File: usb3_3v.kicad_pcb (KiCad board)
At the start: 2 copper layers, 6 parts, among them J1 USB-MICRO-B, P1 +3.3, P2 GND, U1 AAT3221 / MIC5504

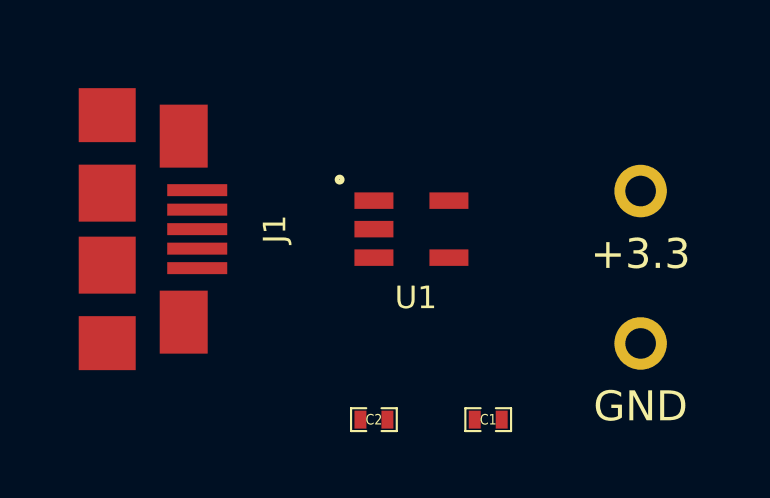
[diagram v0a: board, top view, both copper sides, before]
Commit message: - pcb done, add gerbers
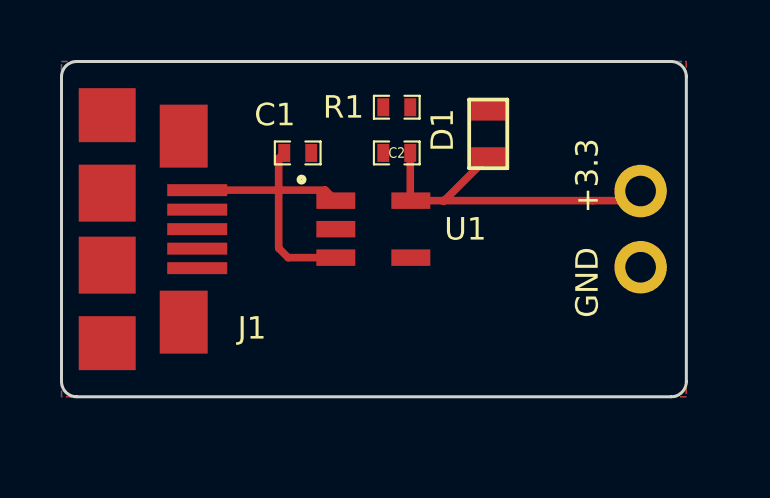
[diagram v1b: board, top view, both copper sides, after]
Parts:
- added D1: LED, SM0603, F.Cu at (227.3, 141.6)
- added R1: 1K, SM0402_r, F.Cu at (224.3, 140.7)
- moved C1 10.9 mm to (221.0, 142.2)
- moved C2 8.92 mm to (224.3, 142.2), turned to 180 degrees
- moved P2 2.54 mm to (232.4, 146.1), turned to 270 degrees
- moved U1 1.27 mm to (222.2, 144.8)
- turned P1 to 270 degrees
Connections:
- C1 pad 1: GND -> /+5v
- J1 pad 1: GND -> /+5v
- U1 pad 1: GND -> /+5v
- U1 pad 2: (no net) -> GND
- U1 pad 3: GND -> /+5v
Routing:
- net /+3.3v: track 0.00 -> 11.5 mm
- net /+5v: track 0.00 -> 10.1 mm
- added copper zone on B.Cu, net GND
- added copper zone on F.Cu, net GND
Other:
- board outline added: 20.8 x 11.2 mm
- board text added: "github.com/ noahp/usb3_3v v0.1"
